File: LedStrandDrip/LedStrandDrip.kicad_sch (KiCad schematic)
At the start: 5 parts, among them J1 PJ-102B, J2 Conn_01x01_Pin, J3 Screw_Terminal_01x03, J4 Screw_Terminal_01x02

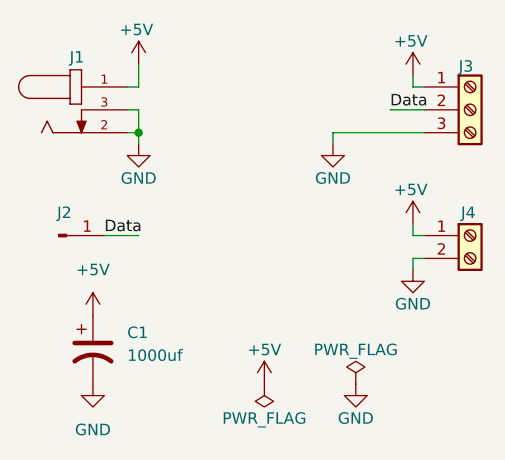
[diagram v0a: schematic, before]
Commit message: incremental updates
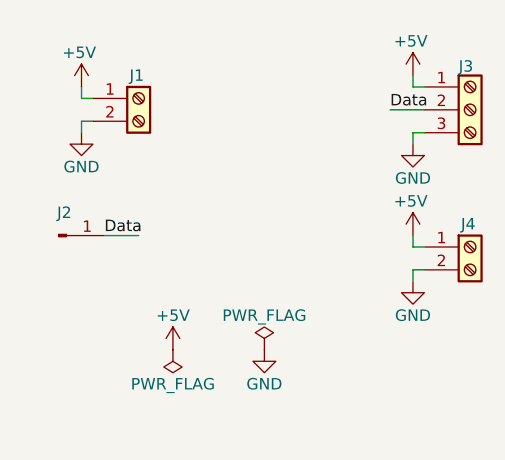
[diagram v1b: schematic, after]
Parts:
- removed C1: 1000uf, Capacitor_THT:CP_Radial_D10.0mm_P5.00mm, symbol Device:C_Polarized_US
- removed J1: PJ-102B, MyTerminalBlock:CUI_PJ-102B, symbol PJ-102B:PJ-102B
- added J4: Screw_Terminal_01x02, MyTerminalBlock:PHOENIX - TERM BLK 2P SIDE ENT 5.08MM PCB, symbol Connector:Screw_Terminal_01x02
- renumbered J4 to J1
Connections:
- net +5V: now also J4.1 (Pin_1)
- net GND: now also J4.2 (Pin_2)
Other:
- moved on the sheet: J1
